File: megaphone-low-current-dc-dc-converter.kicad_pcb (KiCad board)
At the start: 2 copper layers, 13.8 x 21.9 mm, 9 parts, among them U1 TPS631000DRLR

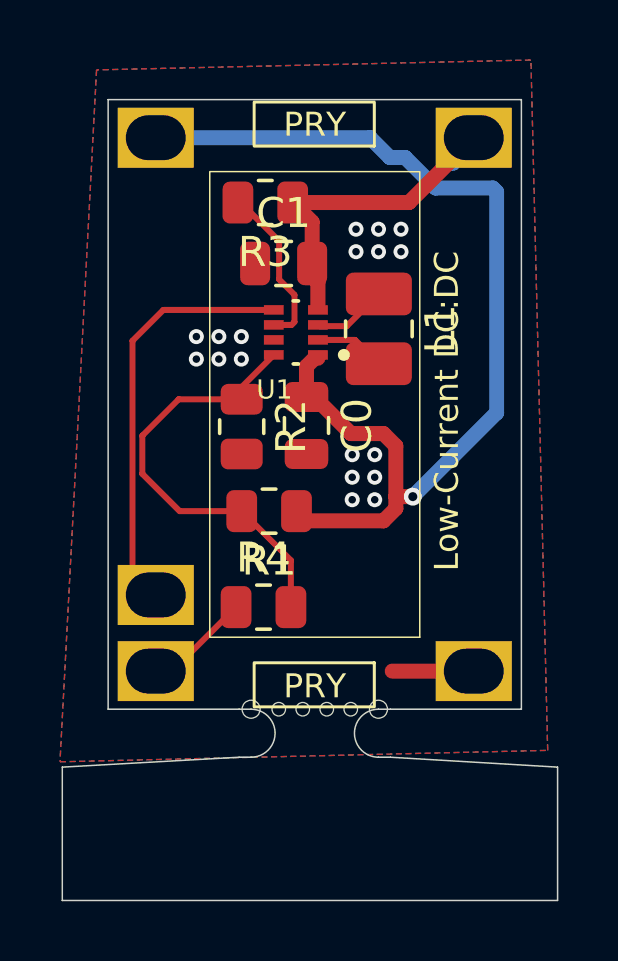
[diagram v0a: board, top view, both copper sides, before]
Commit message: finish PCB layout
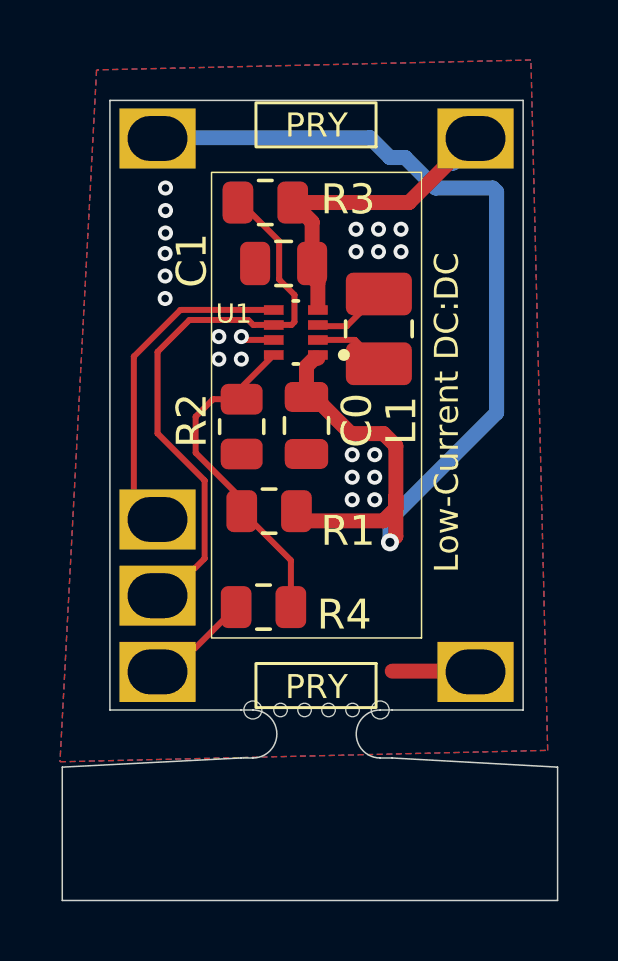
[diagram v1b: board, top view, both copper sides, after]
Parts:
- removed M1: ~, MegaCastle:MegaCastle2x8-Module-I7.0x15.5-M8183-PANEL-NIBBLE
- added M2: ~, MegaCastle:MegaCastle2x8-Module-I7.0x15.5-M8187-PANEL-NIBBLE, B.Cu at (120.2, 75.6)
- U1: value TPS631000DRLR -> U1=TPS631000DRLR
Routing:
- net MODE: track 5.54 -> 21.8 mm
- net EN: track 15.1 -> 11.1 mm
- net Net-(U1-FB): track 14.7 -> 11.4 mm
- net VOUT: track 35.8 -> 38.6 mm
- net GND: track 2.72 -> 3.85 mm, vias 18 -> 22
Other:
- board text added: "1V8 SEL"
- board text added: "MODE"
- board text added: "R20250222"
- board text added: "Tie for 1V8"
- board text removed: "R20250222 github.com /gardners"
